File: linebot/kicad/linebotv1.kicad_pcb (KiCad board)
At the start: 2 copper layers, 43.2 x 61.1 mm, 18 parts, among them IC1 ATTINY85-P, P1 Motor, P2 Motor, SW1 Switch, U1 Phototransistor, U2 Phototransistor, U3 BC337, U4 BC337

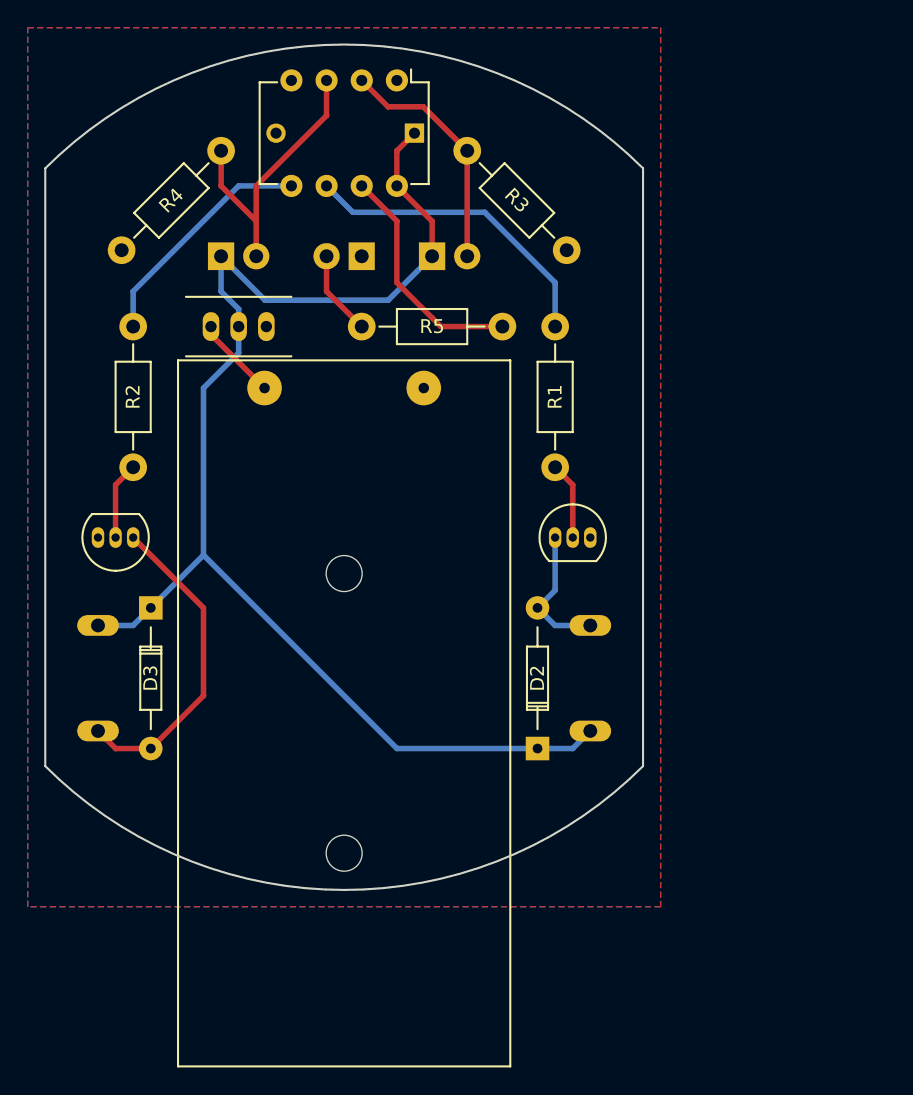
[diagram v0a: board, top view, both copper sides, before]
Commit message: Boards updated
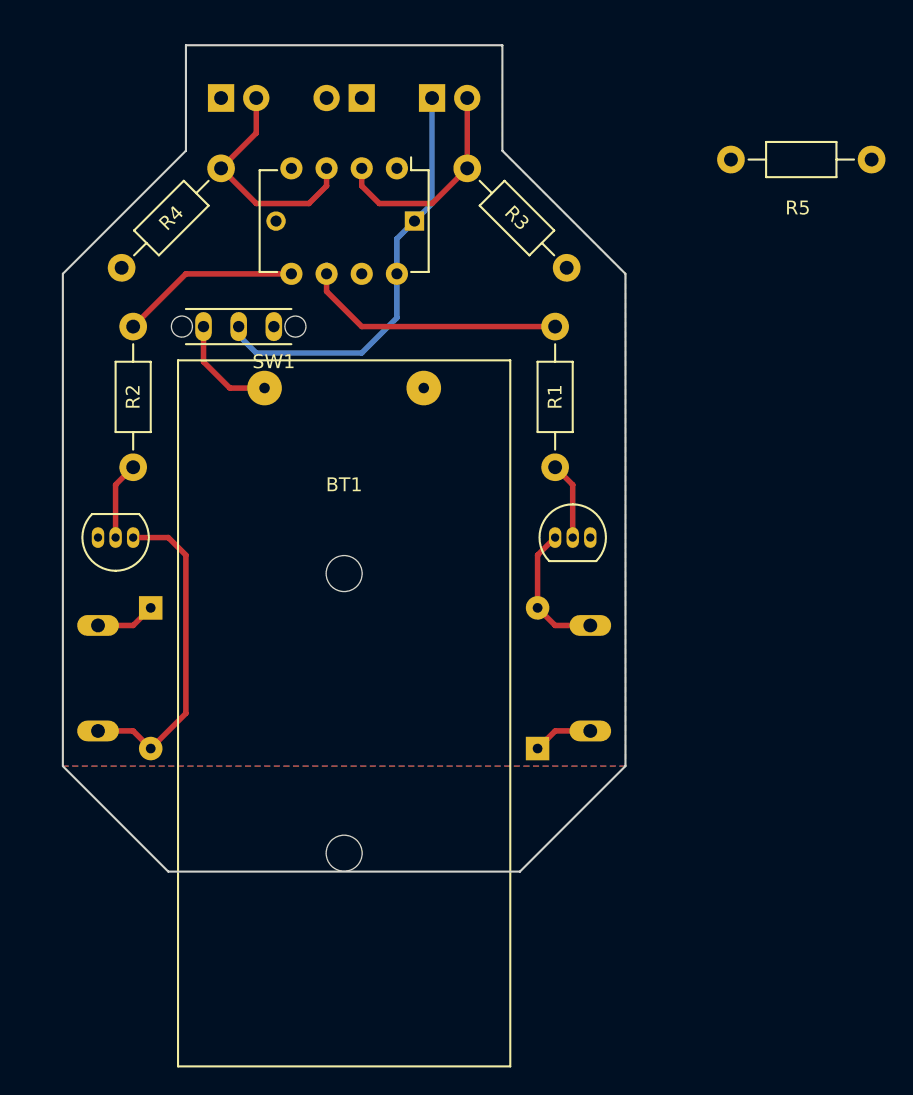
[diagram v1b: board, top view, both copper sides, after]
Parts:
- D2, D3: moved to B.Cu
- SW1: footprint Schiebeschalter -> schiebeschalter:Schiebeschalter
- moved R5 29.3 mm to (190.5, 83.2)
- moved D1 11.4 mm to (153.7, 78.7)
- moved U1 11.4 mm to (158.8, 78.7)
- moved U2 11.4 mm to (143.5, 78.7)
- moved C1 6.35 mm to (157.5, 87.6)
- moved IC1 6.35 mm to (156.2, 83.8)
- moved R3 1.27 mm to (161.3, 83.8)
- moved R4 1.27 mm to (143.5, 83.8)
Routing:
- net VCC: track 95.5 -> 39.2 mm
- net Net-(IC1-Pad7): track 17.0 -> 0.00 mm
- net Net-(D1-Pad2): track 6.13 -> 0.00 mm
- net Net-(IC1-Pad3): track 20.9 -> 16.6 mm
- net Net-(IC1-Pad5): track 17.1 -> 13.0 mm
- net Net-(IC1-Pad6): track 22.6 -> 19.5 mm
- net Net-(IC1-Pad2): track 17.3 -> 15.5 mm
- net Net-(BT1-Pad1): track 6.04 -> 7.74 mm
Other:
- board size 43.2 x 61.1 mm -> 40.6 x 59.7 mm
